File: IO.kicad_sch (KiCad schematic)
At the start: 3 parts, among them J5 02x12, J6 DEBUG_INTERFACE_L, J7 DEBUG_INTERFACE_R

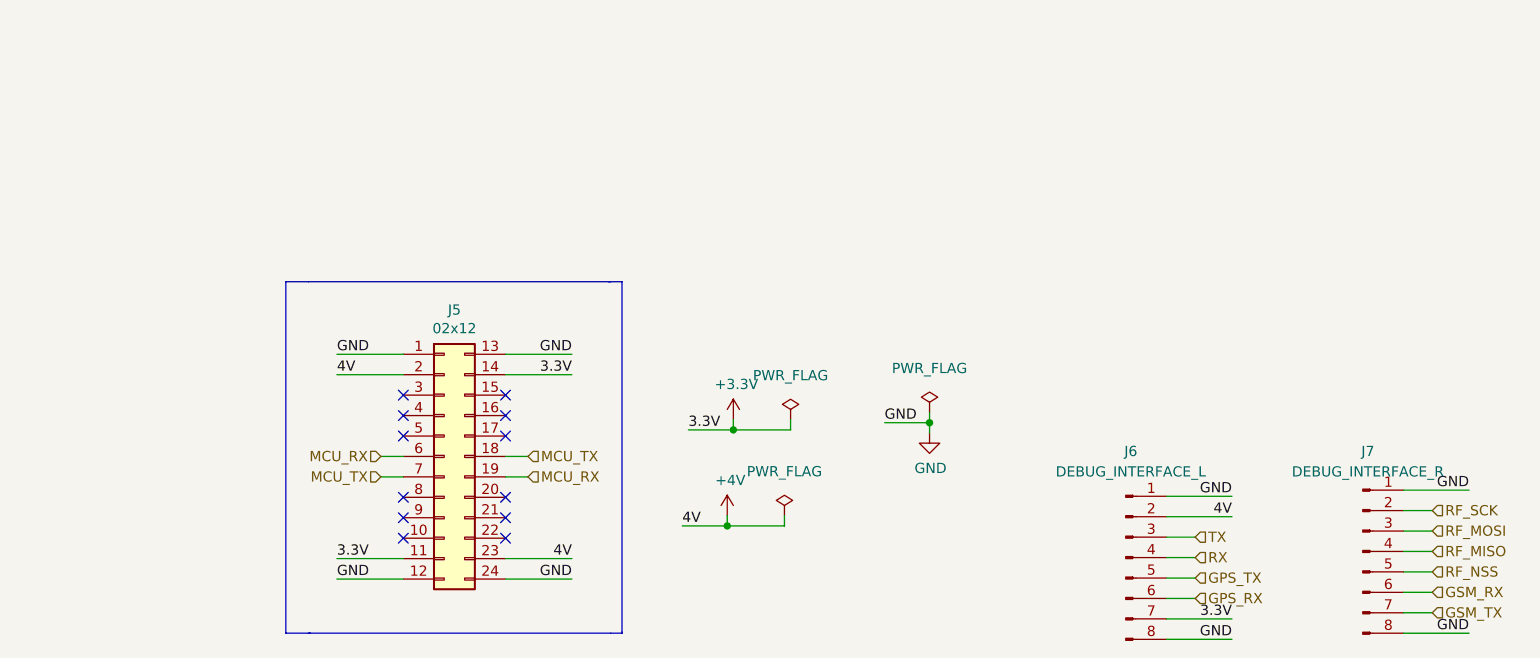
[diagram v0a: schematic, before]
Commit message: KiCad 0.3v
Improved aesthetics.
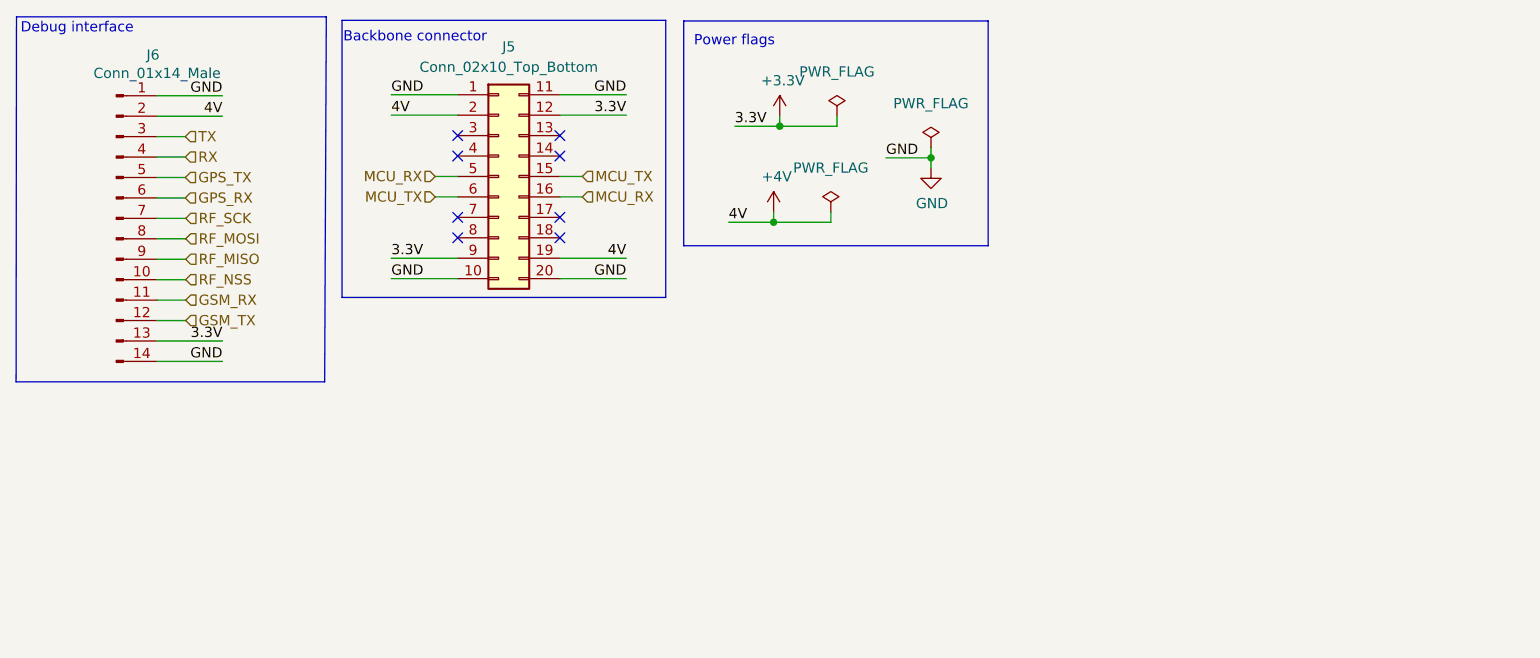
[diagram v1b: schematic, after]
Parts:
- removed J5: 02x12, LOCAL:SAMTEC-SSW-112-02-X-D-RA, symbol Connector_Generic:Conn_02x12_Top_Bottom
- removed J6: DEBUG_INTERFACE_L, symbol Connector:Conn_01x08_Male
- removed J7: DEBUG_INTERFACE_R, symbol Connector:Conn_01x08_Male
- added J5: Conn_02x10_Top_Bottom, Connector_PinHeader_2.54mm:PinHeader_2x20_P2.54mm_Horizontal, symbol Connector_Generic:Conn_02x10_Top_Bottom
- added J6: Conn_01x14_Male, Connector_PinHeader_2.54mm:PinHeader_1x14_P2.54mm_Horizontal, symbol Connector:Conn_01x14_Male
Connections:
- net +3V3: now also J5.12 (Pin_12), J5.9 (Pin_9), J6.13 (Pin_13)
- net +4V: now also J5.19 (Pin_19), J5.2 (Pin_2), J6.2 (Pin_2)
- net GND: now also J5.1 (Pin_1), J5.10 (Pin_10), J5.11 (Pin_11), J5.20 (Pin_20), J6.1 (Pin_1), J6.14 (Pin_14)
- net GPS_RX: now also J6.6 (Pin_6)
- net GPS_TX: now also J6.5 (Pin_5)
- net GSM_RX: now also J6.11 (Pin_11)
- net GSM_TX: now also J6.12 (Pin_12)
- net MCU_RX: now also J5.16 (Pin_16), J5.5 (Pin_5)
- net MCU_TX: now also J5.15 (Pin_15), J5.6 (Pin_6)
- net RF_MISO: now also J6.9 (Pin_9)
- net RF_MOSI: now also J6.8 (Pin_8)
- net RF_NSS: now also J6.10 (Pin_10)
- net RF_SCK: now also J6.7 (Pin_7)
- net RX: now also J6.4 (Pin_4)
- net TX: now also J6.3 (Pin_3)
- no-connect marks 12 -> 8
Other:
- note added: "Backbone connector"
- note added: "Debug interface"
- note added: "Power flags"
